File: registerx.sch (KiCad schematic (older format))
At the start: 6 parts, among them U32 74LS245, U33 74LS173, U34 74LS173, U35 74LS245, U36 74LS173, U37 74LS173

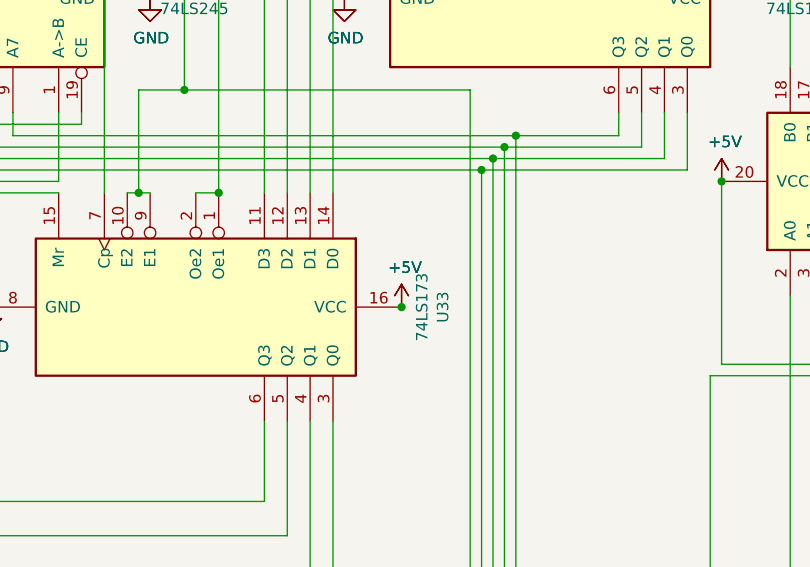
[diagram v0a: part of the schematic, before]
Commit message: fixed more errors
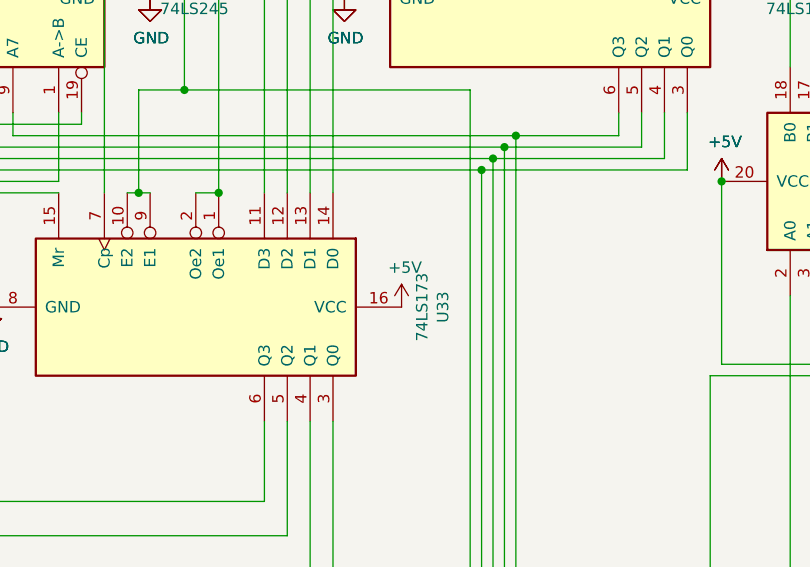
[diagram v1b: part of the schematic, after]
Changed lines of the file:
@@
 	2000 4000 2000 6100
 Wire Wire Line
-	4100 6100 4100 5350
-Wire Wire Line
-	4000 5350 4000 6000
-Wire Wire Line
 	2100 6000 2100 4000
 Wire Wire Line
 	2200 4000 2200 5850
-Wire Wire Line
-	3900 5850 3900 5350
-Wire Wire Line
-	3800 5350 3800 5700
 Wire Wire Line
 	2300 5700 2300 4000
@@
 F 3 "" H 4150 3500 50  0001 C CNN
 	1    4150 3500
-	1    0    0    -1
-$EndComp
-$Comp
-L 16bitCpu-rescue:+5V-power #PWR?
-U 1 1 62492024
-P 4400 4850
-AR Path="/62492024" Ref="#PWR?"  Part="1"
-AR Path="/5F67C726/62492024" Ref="#PWR?"  Part="1"
-AR Path="/5F70885A/62492024" Ref="#PWR?"  Part="1"
-AR Path="/5F733C5E/62492024" Ref="#PWR?"  Part="1"
-AR Path="/602D4838/62492024" Ref="#PWR?"  Part="1"
-AR Path="/603B00C8/62492024" Ref="#PWR?"  Part="1"
-AR Path="/603B766D/62492024" Ref="#PWR?"  Part="1"
-AR Path="/5F74778C/62492024" Ref="#PWR?"  Part="1"
-AR Path="/5FB94562/62492024" Ref="#PWR?"  Part="1"
-AR Path="/61DF6CC7/62492024" Ref="#PWR0137"  Part="1"
-F 0 "#PWR0137" H 4400 4700 50  0001 C CNN
-F 1 "+5V" H 4415 5023 50  0000 C CNN
-F 2 "" H 4400 4850 50  0001 C CNN
-F 3 "" H 4400 4850 50  0001 C CNN
-	1    4400 4850
 	1    0    0    -1
 $EndComp
@@
 Wire Wire Line
 	6500 8600 10200 8600
-$Comp
-L 16bitCpu-rescue:74LS173-74xx U?
-U 1 1 6249200F
-P 3500 4850
-AR Path="/6249200F" Ref="U?"  Part="1"
-AR Path="/5F67C726/6249200F" Ref="U?"  Part="1"
-AR Path="/5F70885A/6249200F" Ref="U?"  Part="1"
-AR Path="/5F733C5E/6249200F" Ref="U?"  Part="1"
-AR Path="/602D4838/6249200F" Ref="U?"  Part="1"
-AR Path="/603B00C8/6249200F" Ref="U?"  Part="1"
-AR Path="/603B766D/6249200F" Ref="U?"  Part="1"
-AR Path="/5F74778C/6249200F" Ref="U?"  Part="1"
-AR Path="/5FB94562/6249200F" Ref="U?"  Part="1"
-AR Path="/61DF6CC7/6249200F" Ref="U33"  Part="1"
-F 0 "U33" H 3500 5931 50  0000 C CNN
-F 1 "74LS173" H 3500 5840 50  0000 C CNN
-F 2 "Package_DIP:DIP-16_W7.62mm" H 3500 4850 50  0001 C CNN
-F 3 "http://www.ti.com/lit/gpn/sn74LS173" H 3500 4850 50  0001 C CNN
-	1    3500 4850
-	0    1    1    0
-$EndComp
 $Comp
 L 16bitCpu-rescue:74LS245-74xx U?
@@
 F 3 "" H 1700 3500 50  0001 C CNN
 	1    1700 3500
-	1    0    0    -1
-$EndComp
-$Comp
-L 16bitCpu-rescue:+5V-power #PWR?
-U 1 1 5F6AAC53
-P 4400 4850
-AR Path="/5F6AAC53" Ref="#PWR?"  Part="1"
-AR Path="/5F67C726/5F6AAC53" Ref="#PWR?"  Part="1"
-AR Path="/5F70885A/5F6AAC53" Ref="#PWR?"  Part="1"
-AR Path="/5F733C5E/5F6AAC53" Ref="#PWR?"  Part="1"
-AR Path="/602D4838/5F6AAC53" Ref="#PWR?"  Part="1"
-AR Path="/603B00C8/5F6AAC53" Ref="#PWR?"  Part="1"
-AR Path="/603B766D/5F6AAC53" Ref="#PWR?"  Part="1"
-AR Path="/5F74778C/5F6AAC53" Ref="#PWR?"  Part="1"
-AR Path="/5FB94562/5F6AAC53" Ref="#PWR?"  Part="1"
-AR Path="/61DF6CC7/5F6AAC53" Ref="#PWR0136"  Part="1"
-F 0 "#PWR0136" H 4400 4700 50  0001 C CNN
-F 1 "+5V" H 4415 5023 50  0000 C CNN
-F 2 "" H 4400 4850 50  0001 C CNN
-F 3 "" H 4400 4850 50  0001 C CNN
-	1    4400 4850
 	1    0    0    -1
 $EndComp
@@
 Text HLabel 1300 2250 0    50   3State ~ 0
 Bus14
-Connection ~ 3600 4350
-Connection ~ 4400 4850
-Connection ~ 2600 4850
 Wire Wire Line
 	10250 3050 10250 7750
@@
 	9450 7600 1150 7600
 Connection ~ 9450 4900
+Connection ~ 2600 4850
+Connection ~ 3600 4350
+Wire Wire Line
+	4100 6100 4100 5350
+Wire Wire Line
+	4000 5350 4000 6000
+Wire Wire Line
+	3900 5850 3900 5350
+Wire Wire Line
+	3800 5350 3800 5700
+$Comp
+L 16bitCpu-rescue:74LS173-74xx U?
+U 1 1 6249200F
+P 3500 4850
+AR Path="/6249200F" Ref="U?"  Part="1"
+AR Path="/5F67C726/6249200F" Ref="U?"  Part="1"
+AR Path="/5F70885A/6249200F" Ref="U?"  Part="1"
+AR Path="/5F733C5E/6249200F" Ref="U?"  Part="1"
+AR Path="/602D4838/6249200F" Ref="U?"  Part="1"
+AR Path="/603B00C8/6249200F" Ref="U?"  Part="1"
+AR Path="/603B766D/6249200F" Ref="U?"  Part="1"
+AR Path="/5F74778C/6249200F" Ref="U?"  Part="1"
+AR Path="/5FB94562/6249200F" Ref="U?"  Part="1"
+AR Path="/61DF6CC7/6249200F" Ref="U33"  Part="1"
+F 0 "U33" H 3500 5931 50  0000 C CNN
+F 1 "74LS173" H 3500 5840 50  0000 C CNN
+F 2 "Package_DIP:DIP-16_W7.62mm" H 3500 4850 50  0001 C CNN
+F 3 "http://www.ti.com/lit/gpn/sn74LS173" H 3500 4850 50  0001 C CNN
+	1    3500 4850
+	0    1    1    0
+$EndComp
+$Comp
+L 16bitCpu-rescue:+5V-power #PWR?
+U 1 1 62492024
+P 4400 4850
+AR Path="/62492024" Ref="#PWR?"  Part="1"
+AR Path="/5F67C726/62492024" Ref="#PWR?"  Part="1"
+AR Path="/5F70885A/62492024" Ref="#PWR?"  Part="1"
+AR Path="/5F733C5E/62492024" Ref="#PWR?"  Part="1"
+AR Path="/602D4838/62492024" Ref="#PWR?"  Part="1"
+AR Path="/603B00C8/62492024" Ref="#PWR?"  Part="1"
+AR Path="/603B766D/62492024" Ref="#PWR?"  Part="1"
+AR Path="/5F74778C/62492024" Ref="#PWR?"  Part="1"
+AR Path="/5FB94562/62492024" Ref="#PWR?"  Part="1"
+AR Path="/61DF6CC7/62492024" Ref="#PWR0137"  Part="1"
+F 0 "#PWR0137" H 4400 4700 50  0001 C CNN
+F 1 "+5V" H 4415 5023 50  0000 C CNN
+F 2 "" H 4400 4850 50  0001 C CNN
+F 3 "" H 4400 4850 50  0001 C CNN
+	1    4400 4850
+	1    0    0    -1
+$EndComp
 $EndSCHEMATC
